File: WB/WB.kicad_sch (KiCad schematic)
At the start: 47 parts, among them J1 Conn_01x04, J2 Conn_01x04, J3 Conn_01x04, J4 Conn_01x04, J5 Pump, J6 Actuator, J7 Actuator, J8 Screw_Terminal_01x02, M1 Fan, Q1 Q_NMOS_GDS, Q2 Q_NMOS_GDS, Q3 Q_NMOS_GDS, Q4 Q_NMOS_GDS, Q5 Q_NMOS_GDS, Q6 Q_NMOS_GDS, Q7 Q_NMOS_GDS, Q8 Q_NPN_ECB, SW1 SW_Push, SW2 SW_Push, SW3 SW_Push, SW4 SW_Push, SW5 SW_Push, SW6 SW_Push, U1 74HC165, U2 74HC595, U3 TB6643KQ, U4 Arduino_Micro

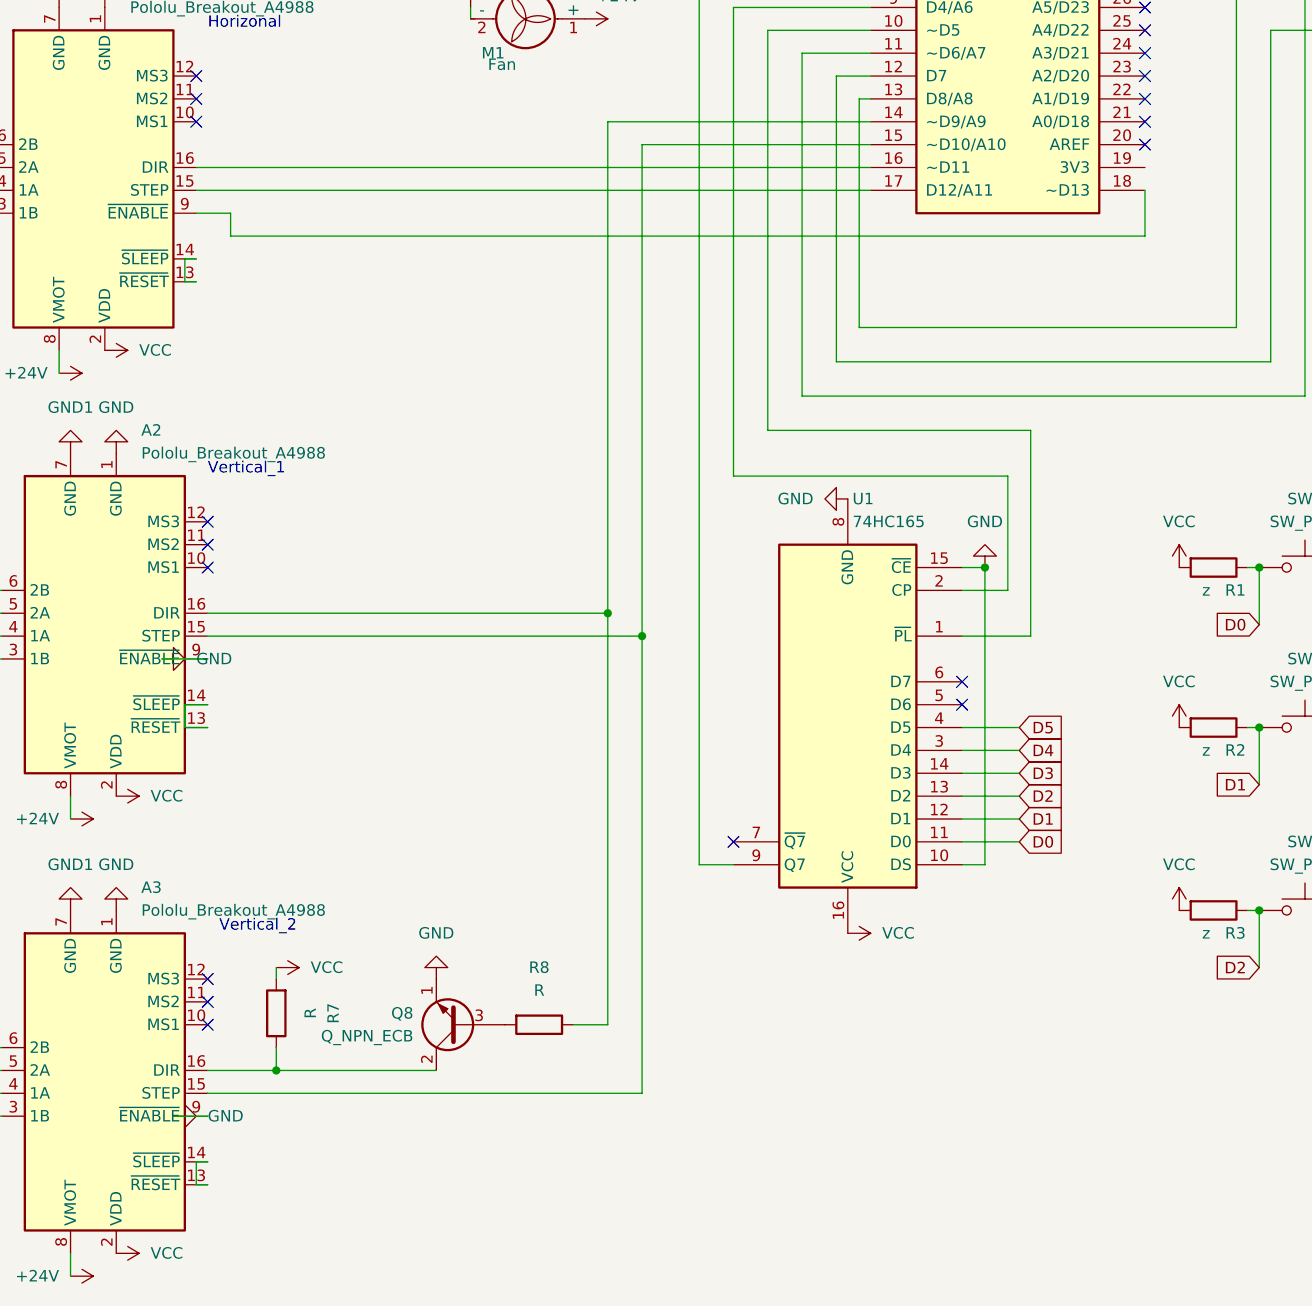
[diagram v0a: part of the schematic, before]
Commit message: 回路周りのファイル
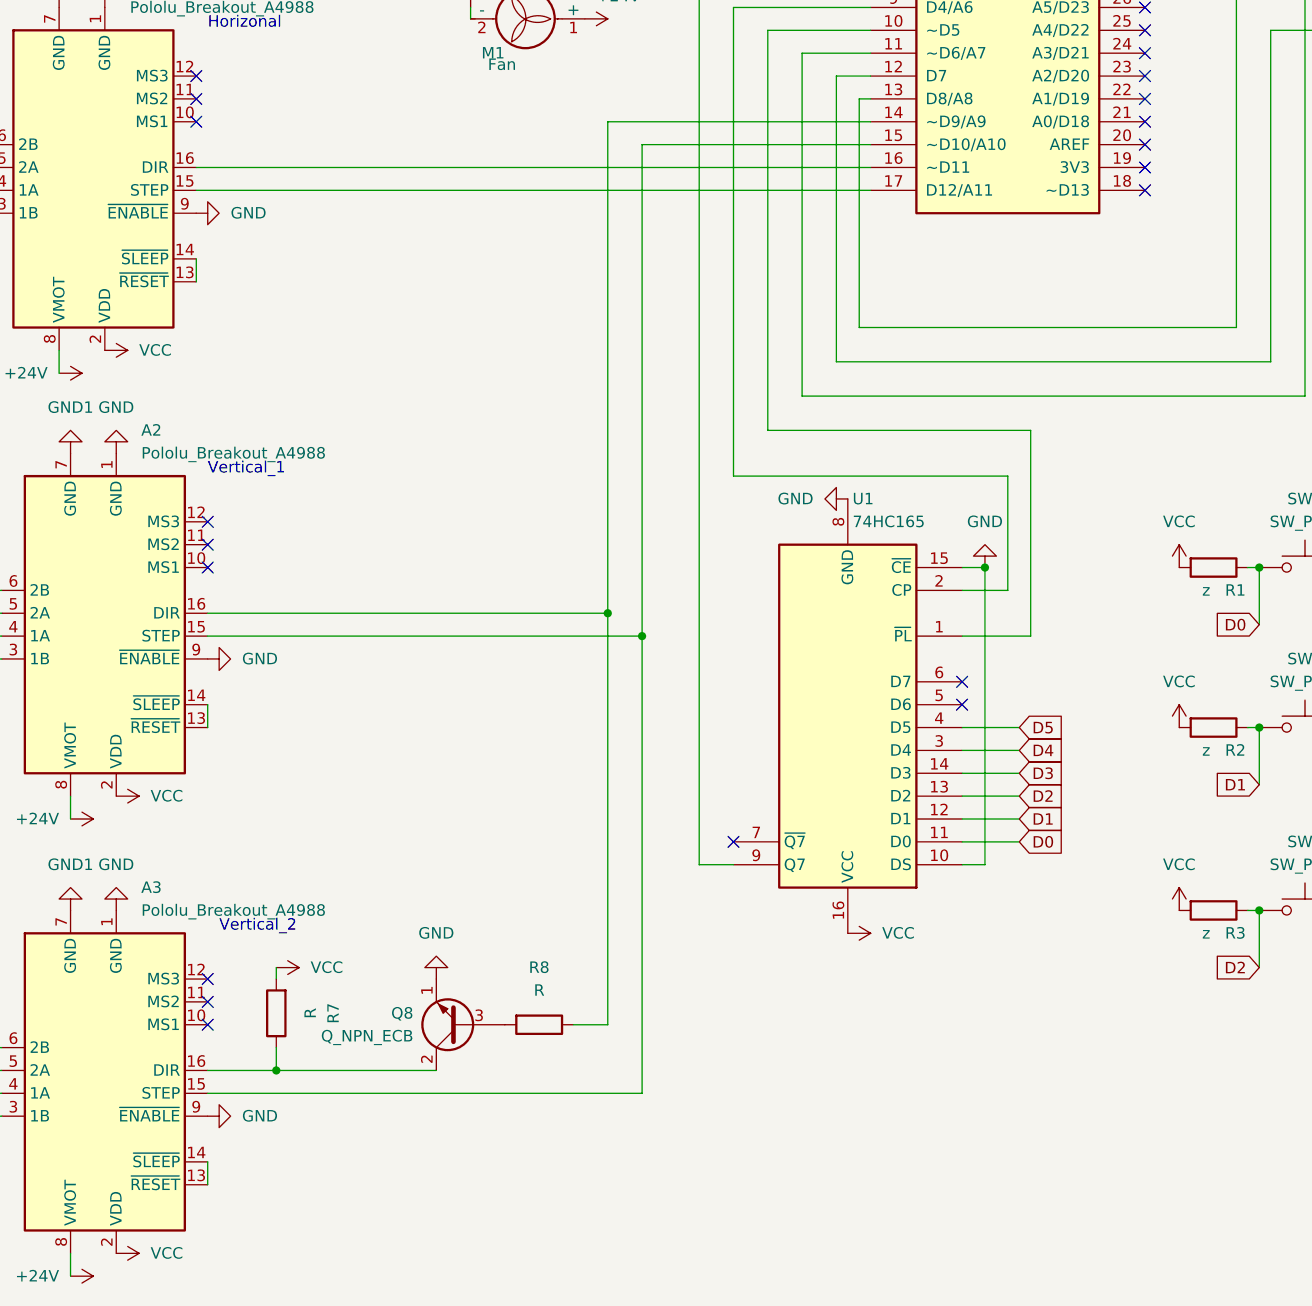
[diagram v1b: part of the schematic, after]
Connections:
- net GND: now also A1.9 (~{ENABLE})
- net at U4.18 (~D13): no longer A1.9 (~{ENABLE})
- no-connect marks 31 -> 33
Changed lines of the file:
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@@
   (no_connect (at 54.61 49.53))
   (no_connect (at 54.61 46.99))
+  (no_connect (at 160.02 59.69))
+  (no_connect (at 160.02 57.15))
   (no_connect (at 160.02 34.29))
   (no_connect (at 160.02 39.37))
@@
     (stroke (width 0) (type default) (color 0 0 0 0))
   )
-  (wire (pts (xy 58.42 64.77) (xy 160.02 64.77))
-    (stroke (width 0) (type default) (color 0 0 0 0))
-  )
   (wire (pts (xy 232.41 31.75) (xy 232.41 100.33))
     (stroke (width 0) (type default) (color 0 0 0 0))
   )
-  (wire (pts (xy 53.34 67.31) (xy 53.34 69.85))
+  (wire (pts (xy 54.61 67.31) (xy 54.61 69.85))
     (stroke (width 0) (type default) (color 0 0 0 0))
   )
@@
     (stroke (width 0) (type default) (color 0 0 0 0))
   )
-  (wire (pts (xy 55.88 162.56) (xy 52.07 162.56))
-    (stroke (width 0) (type default) (color 0 0 0 0))
-  )
   (wire (pts (xy 114.3 39.37) (xy 129.54 39.37))
     (stroke (width 0) (type default) (color 0 0 0 0))
   )
-  (wire (pts (xy 53.34 119.38) (xy 55.88 119.38))
-    (stroke (width 0) (type default) (color 0 0 0 0))
-  )
   (wire (pts (xy 199.39 119.38) (xy 200.66 119.38))
     (stroke (width 0) (type default) (color 0 0 0 0))
@@
     (stroke (width 0) (type default) (color 0 0 0 0))
   )
-  (wire (pts (xy 55.88 116.84) (xy 53.34 116.84))
-    (stroke (width 0) (type default) (color 0 0 0 0))
-  )
   (wire (pts (xy 30.48 71.12) (xy 30.48 54.61))
     (stroke (width 0) (type default) (color 0 0 0 0))
   )
-  (wire (pts (xy 160.02 64.77) (xy 160.02 59.69))
-    (stroke (width 0) (type default) (color 0 0 0 0))
-  )
   (wire (pts (xy 248.92 69.85) (xy 255.27 69.85))
     (stroke (width 0) (type default) (color 0 0 0 0))
@@
     (stroke (width 0) (type default) (color 0 0 0 0))
   )
-  (wire (pts (xy 54.61 67.31) (xy 53.34 67.31))
-    (stroke (width 0) (type default) (color 0 0 0 0))
-  )
   (wire (pts (xy 139.7 124.46) (xy 146.05 124.46))
     (stroke (width 0) (type default) (color 0 0 0 0))
@@
     (stroke (width 0) (type default) (color 0 0 0 0))
   )
-  (wire (pts (xy 53.34 69.85) (xy 54.61 69.85))
-    (stroke (width 0) (type default) (color 0 0 0 0))
-  )
   (wire (pts (xy 250.19 139.7) (xy 254 139.7))
     (stroke (width 0) (type default) (color 0 0 0 0))
   )
-  (wire (pts (xy 58.42 62.23) (xy 54.61 62.23))
-    (stroke (width 0) (type default) (color 0 0 0 0))
-  )
   (wire (pts (xy 237.49 36.83) (xy 237.49 64.77))
     (stroke (width 0) (type default) (color 0 0 0 0))
@@
     (stroke (width 0) (type default) (color 0 0 0 0))
   )
-  (wire (pts (xy 55.88 167.64) (xy 54.61 167.64))
-    (stroke (width 0) (type default) (color 0 0 0 0))
-  )
   (wire (pts (xy 241.3 41.91) (xy 220.98 41.91))
     (stroke (width 0) (type default) (color 0 0 0 0))
@@
     (stroke (width 0) (type default) (color 0 0 0 0))
   )
-  (wire (pts (xy 54.61 170.18) (xy 55.88 170.18))
-    (stroke (width 0) (type default) (color 0 0 0 0))
-  )
   (wire (pts (xy 224.79 142.24) (xy 234.95 142.24))
     (stroke (width 0) (type default) (color 0 0 0 0))
@@
     (stroke (width 0) (type default) (color 0 0 0 0))
   )
-  (wire (pts (xy 53.34 116.84) (xy 53.34 119.38))
+  (wire (pts (xy 55.88 116.84) (xy 55.88 119.38))
     (stroke (width 0) (type default) (color 0 0 0 0))
   )
@@
     (stroke (width 0) (type default) (color 0 0 0 0))
   )
-  (wire (pts (xy 55.88 111.76) (xy 50.8 111.76))
-    (stroke (width 0) (type default) (color 0 0 0 0))
-  )
   (wire (pts (xy 262.89 149.86) (xy 266.7 149.86))
     (stroke (width 0) (type default) (color 0 0 0 0))
@@
     (stroke (width 0) (type default) (color 0 0 0 0))
   )
-  (wire (pts (xy 58.42 64.77) (xy 58.42 62.23))
-    (stroke (width 0) (type default) (color 0 0 0 0))
-  )
   (wire (pts (xy 248.92 87.63) (xy 255.27 87.63))
     (stroke (width 0) (type default) (color 0 0 0 0))
@@
     (stroke (width 0) (type default) (color 0 0 0 0))
   )
-  (wire (pts (xy 54.61 167.64) (xy 54.61 170.18))
+  (wire (pts (xy 55.88 167.64) (xy 55.88 170.18))
     (stroke (width 0) (type default) (color 0 0 0 0))
   )
@@
     (pin "1")
   )
+  (symbol (lib_id "power:GND") (at 54.61 62.23 90) (unit 1)
+    (in_bom yes) (on_board yes) (fields_autoplaced)
+    (property "Reference" "#PWR?" (id 0) (at 60.96 62.23 0)
+      (effects (font (size 1.27 1.27)) hide)
+    )
+    (property "Value" "GND" (id 1) (at 58.42 62.2299 90)
+      (effects (font (size 1.27 1.27)) (justify right))
+    )
+    (property "Footprint" "" (id 2) (at 54.61 62.23 0)
+      (effects (font (size 1.27 1.27)) hide)
+    )
+    (property "Datasheet" "" (id 3) (at 54.61 62.23 0)
+      (effects (font (size 1.27 1.27)) hide)
+    )
+    (pin "1")
+  )
   (symbol (lib_id "Device:Q_NMOS_GDS") (at 246.38 100.33 0) (unit 1)
     (in_bom yes) (on_board yes)
@@
     (pin "3")
   )
-  (symbol (lib_id "power:GND") (at 50.8 111.76 90) (unit 1)
-    (in_bom yes) (on_board yes) (fields_autoplaced)
-    (property "Reference" "#PWR014" (id 0) (at 57.15 111.76 0)
-      (effects (font (size 1.27 1.27)) hide)
-    )
-    (property "Value" "GND" (id 1) (at 54.61 111.7599 90)
-      (effects (font (size 1.27 1.27)) (justify right))
-    )
-    (property "Footprint" "" (id 2) (at 50.8 111.76 0)
-      (effects (font (size 1.27 1.27)) hide)
-    )
-    (property "Datasheet" "" (id 3) (at 50.8 111.76 0)
+  (symbol (lib_id "power:GND") (at 55.88 111.76 90) (unit 1)
+    (in_bom yes) (on_board yes) (fields_autoplaced)
+    (property "Reference" "#PWR014" (id 0) (at 62.23 111.76 0)
+      (effects (font (size 1.27 1.27)) hide)
+    )
+    (property "Value" "GND" (id 1) (at 59.69 111.7599 90)
+      (effects (font (size 1.27 1.27)) (justify right))
+    )
+    (property "Footprint" "" (id 2) (at 55.88 111.76 0)
+      (effects (font (size 1.27 1.27)) hide)
+    )
+    (property "Datasheet" "" (id 3) (at 55.88 111.76 0)
       (effects (font (size 1.27 1.27)) hide)
     )
@@
     (pin "1")
   )
-  (symbol (lib_id "power:GND") (at 52.07 162.56 90) (unit 1)
-    (in_bom yes) (on_board yes) (fields_autoplaced)
-    (property "Reference" "#PWR0125" (id 0) (at 58.42 162.56 0)
-      (effects (font (size 1.27 1.27)) hide)
-    )
-    (property "Value" "GND" (id 1) (at 55.88 162.5599 90)
-      (effects (font (size 1.27 1.27)) (justify right))
-    )
-    (property "Footprint" "" (id 2) (at 52.07 162.56 0)
-      (effects (font (size 1.27 1.27)) hide)
-    )
-    (property "Datasheet" "" (id 3) (at 52.07 162.56 0)
+  (symbol (lib_id "power:GND") (at 55.88 162.56 90) (unit 1)
+    (in_bom yes) (on_board yes) (fields_autoplaced)
+    (property "Reference" "#PWR0125" (id 0) (at 62.23 162.56 0)
+      (effects (font (size 1.27 1.27)) hide)
+    )
+    (property "Value" "GND" (id 1) (at 59.69 162.5599 90)
+      (effects (font (size 1.27 1.27)) (justify right))
+    )
+    (property "Footprint" "" (id 2) (at 55.88 162.56 0)
+      (effects (font (size 1.27 1.27)) hide)
+    )
+    (property "Datasheet" "" (id 3) (at 55.88 162.56 0)
       (effects (font (size 1.27 1.27)) hide)
     )
@@
       (reference "#PWR0130") (unit 1) (value "GND") (footprint "")
     )
+    (path "/26ecf2e6-34aa-44d1-be14-07675bc38317"
+      (reference "#PWR?") (unit 1) (value "GND") (footprint "")
+    )
     (path "/e2dd1781-dd03-47fd-bd79-56dcdb6f3e26"
